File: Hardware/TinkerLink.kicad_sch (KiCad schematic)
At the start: 33 parts, among them J1 Conn_01x06_Pin, Q1 DMN32D2LDF, Q2 MMBT2222A, Q3 SQS411ENW-T1_GE3, Q4 SQS411ENW-T1_GE3, SW1 TS-061D-250D4-P, U1 ESP-01F-2M, U2 INA228, U3 AP63203WU, U4 TPD2EUSB30A

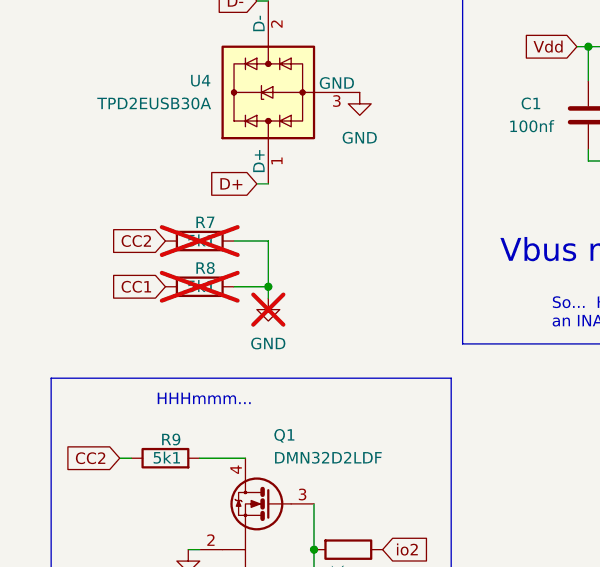
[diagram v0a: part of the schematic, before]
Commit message: Starting to prep for publication
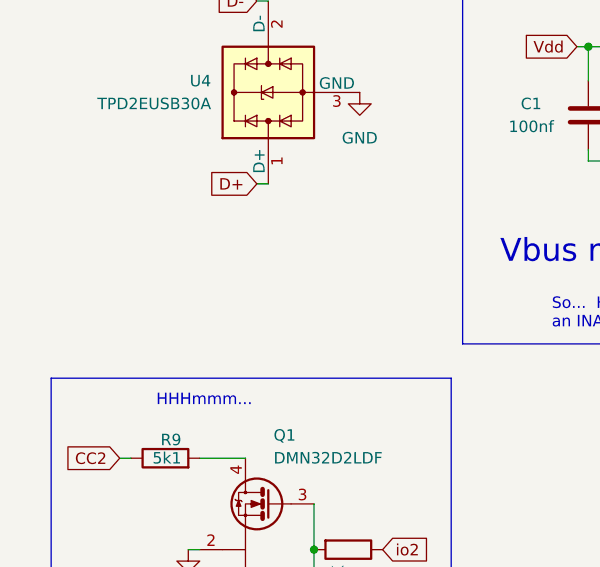
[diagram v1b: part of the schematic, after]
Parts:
- removed R7, R8: 5k1, Resistor_SMD:R_0603_1608Metric, symbol Device:R
- J1, LOGO1, LOGO2: now left out of the parts list
- Q1: LCSC Part (none) -> C672154
- USB2: LCSC Part C5370430, C2765186 -> C5370430
